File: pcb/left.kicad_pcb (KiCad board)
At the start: 2 copper layers, 1 part

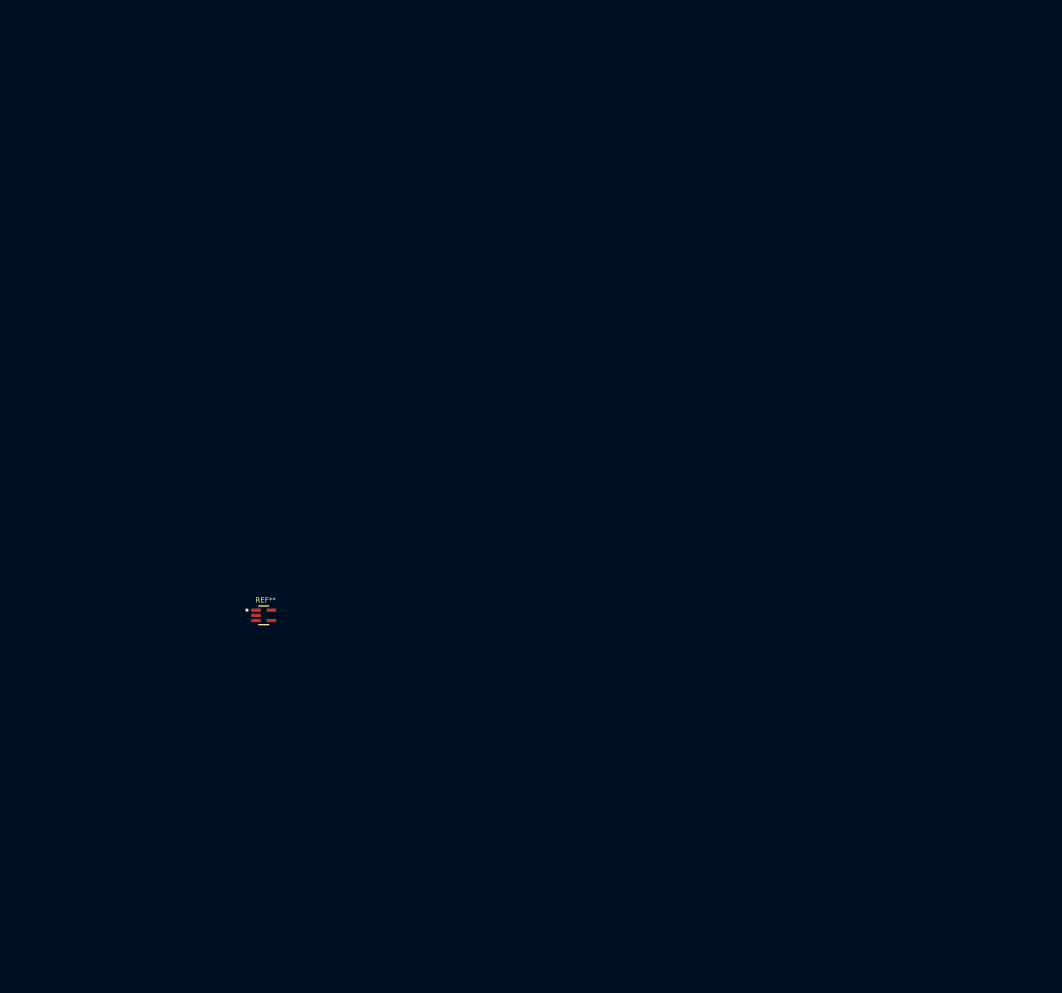
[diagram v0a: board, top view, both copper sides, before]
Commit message: close to finishing layout/placement
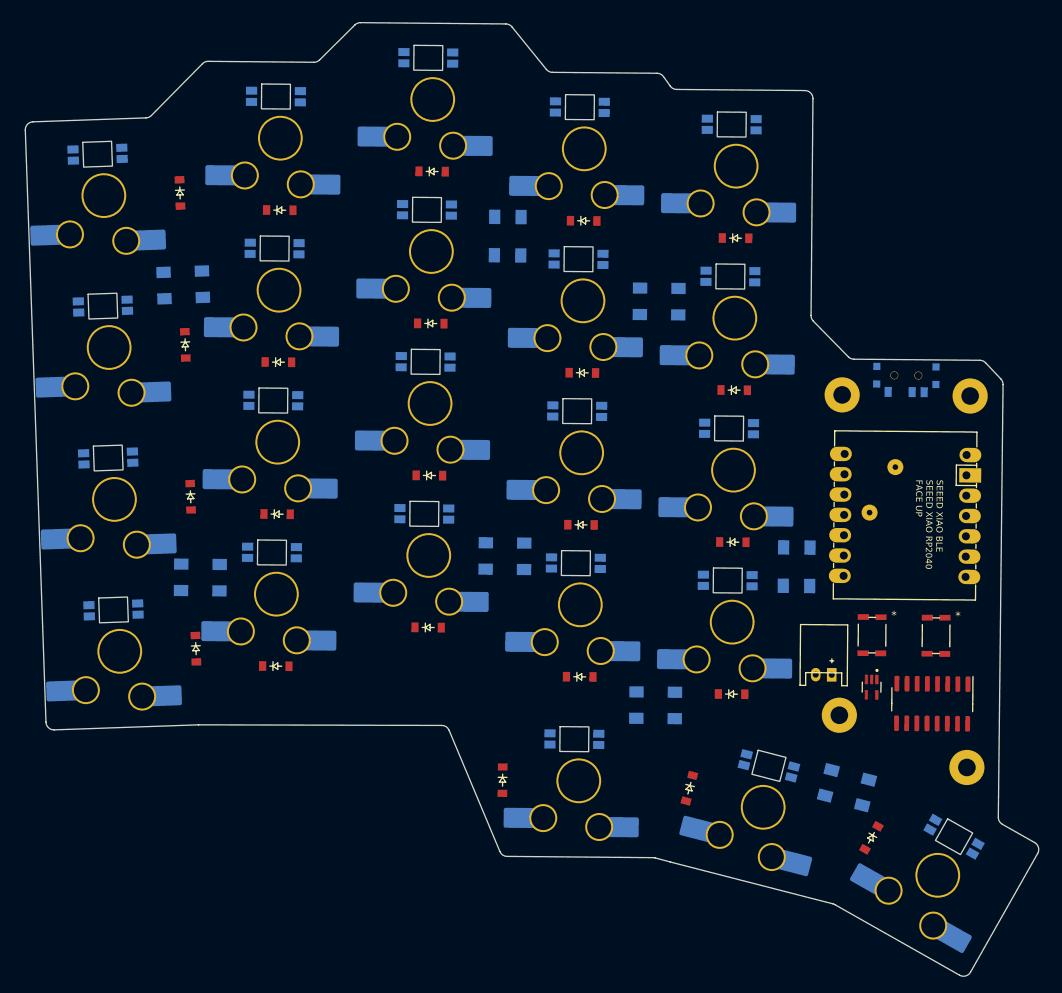
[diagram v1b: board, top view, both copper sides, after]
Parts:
- removed REF**: SOT65P210X110-5N, SN74LV1T34:SOT65P210X110-5N
- added 19.051: 74HC595, SOIC-16_3.9x9.9mm_P1.27mm, F.Cu at (201.6, 106.5)
- added D1: , ComboDiode, F.Cu at (119.5, 101.9)
- added D10: , ComboDiode, F.Cu at (157.7, 84.2)
- added D11: , ComboDiode, F.Cu at (157.8, 65.2)
- added D12: , ComboDiode, F.Cu at (158.0, 46.2)
- added D13: , ComboDiode, F.Cu at (176.5, 105.4)
- added D14: , ComboDiode, F.Cu at (176.6, 86.4)
- added D15: , ComboDiode, F.Cu at (176.8, 67.4)
- added D16: , ComboDiode, F.Cu at (177.0, 48.4)
- added D17: , ComboDiode, F.Cu at (147.9, 116.1)
- added D18: , ComboDiode, F.Cu at (171.2, 117.1)
- added D19: , ComboDiode, F.Cu at (194.0, 123.3)
- added D2: , ComboDiode, F.Cu at (119.7, 82.9)
- added D20: , ComboDiode, F.Cu at (109.5, 99.7)
- added D21: , ComboDiode, F.Cu at (108.9, 80.7)
- added D22: , ComboDiode, F.Cu at (108.2, 61.7)
- added D23: , ComboDiode, F.Cu at (107.5, 42.7)
- added D3: , ComboDiode, F.Cu at (119.8, 63.9)
- added D4: , ComboDiode, F.Cu at (120.0, 44.9)
- added D5: , ComboDiode, F.Cu at (138.5, 97.0)
- added D6: , ComboDiode, F.Cu at (138.7, 78.0)
- added D7: , ComboDiode, F.Cu at (138.9, 59.0)
- added D8: , ComboDiode, F.Cu at (139.0, 40.0)
- added D9: , ComboDiode, F.Cu at (157.5, 103.2)
- added JST1: , JST_PH_S2B-PH-K_02x2.00mm_Angled, F.Cu at (188.0, 102.9)
- added LED1: , ceoloide:led_SK6812mini-e (per-keysingle-side), B.Cu at (99.2, 94.8)
- added LED10: , ceoloide:led_SK6812mini-e (per-keysingle-side), B.Cu at (138.2, 63.8)
- added LED11: , ceoloide:led_SK6812mini-e (per-keysingle-side), B.Cu at (138.4, 44.8)
- added LED12: , ceoloide:led_SK6812mini-e (per-keysingle-side), B.Cu at (138.6, 25.8)
- added LED13: , ceoloide:led_SK6812mini-e (per-keysingle-side), B.Cu at (157.0, 89.0)
- added LED14: , ceoloide:led_SK6812mini-e (per-keysingle-side), B.Cu at (157.2, 70.0)
- added LED15: , ceoloide:led_SK6812mini-e (per-keysingle-side), B.Cu at (157.3, 51.0)
- added LED16: , ceoloide:led_SK6812mini-e (per-keysingle-side), B.Cu at (157.5, 32.0)
- added LED17: , ceoloide:led_SK6812mini-e (per-keysingle-side), B.Cu at (176.0, 91.1)
- added LED18: , ceoloide:led_SK6812mini-e (per-keysingle-side), B.Cu at (176.2, 72.1)
- added LED19: , ceoloide:led_SK6812mini-e (per-keysingle-side), B.Cu at (176.3, 53.1)
- added LED2: , ceoloide:led_SK6812mini-e (per-keysingle-side), B.Cu at (98.6, 75.8)
- added LED20: , ceoloide:led_SK6812mini-e (per-keysingle-side), B.Cu at (176.5, 34.1)
- added LED21: , ceoloide:led_SK6812mini-e (per-keysingle-side), B.Cu at (156.8, 111.0)
- added LED22: , ceoloide:led_SK6812mini-e (per-keysingle-side), B.Cu at (181.1, 114.3)
- added LED23: , ceoloide:led_SK6812mini-e (per-keysingle-side), B.Cu at (204.3, 123.2)
- added LED24: VAL**, WS2812B, B.Cu at (107.9, 54.2)
- added LED25: VAL**, WS2812B, B.Cu at (110.1, 90.8)
- added LED26: VAL**, WS2812B, B.Cu at (148.1, 88.1)
- added LED27: VAL**, WS2812B, B.Cu at (167.0, 106.7)
- added LED28: VAL**, WS2812B, B.Cu at (190.9, 117.0)
- added LED29: VAL**, WS2812B, B.Cu at (167.4, 56.3)
- added LED3: , ceoloide:led_SK6812mini-e (per-keysingle-side), B.Cu at (97.9, 56.8)
- added LED30: VAL**, WS2812B, B.Cu at (184.6, 89.4)
- added LED31: VAL**, WS2812B, B.Cu at (148.5, 48.1)
- added LED4: , ceoloide:led_SK6812mini-e (per-keysingle-side), B.Cu at (97.2, 37.9)
- added LED5: , ceoloide:led_SK6812mini-e (per-keysingle-side), B.Cu at (119.0, 87.6)
- added LED6: , ceoloide:led_SK6812mini-e (per-keysingle-side), B.Cu at (119.2, 68.6)
- added LED7: , ceoloide:led_SK6812mini-e (per-keysingle-side), B.Cu at (119.4, 49.7)
- added LED8: , ceoloide:led_SK6812mini-e (per-keysingle-side), B.Cu at (119.5, 30.7)
- added LED9: , ceoloide:led_SK6812mini-e (per-keysingle-side), B.Cu at (138.1, 82.8)
- added MCU1: , xiao-ble, F.Cu at (198.2, 83.0)
- added PAD1: , MountingHole_2.2mm_M2_Pad, F.Cu at (206.3, 68.1)
- added PAD2: , MountingHole_2.2mm_M2_Pad, F.Cu at (190.3, 67.9)
- added PAD3: , MountingHole_2.2mm_M2_Pad, F.Cu at (205.9, 114.5)
- added PAD4: , MountingHole_2.2mm_M2_Pad, F.Cu at (190.0, 108.0)
- added S1: , ceoloide:switch_gateron_ks27_ks33, B.Cu at (100.0, 100.0)
- added S10: , ceoloide:switch_gateron_ks27_ks33, B.Cu at (138.8, 69.0)
- added S11: , ceoloide:switch_gateron_ks27_ks33, B.Cu at (139.0, 50.0)
- added S12: , ceoloide:switch_gateron_ks27_ks33, B.Cu at (139.1, 31.0)
- added S13: , ceoloide:switch_gateron_ks27_ks33, B.Cu at (157.6, 94.2)
- added S14: , ceoloide:switch_gateron_ks27_ks33, B.Cu at (157.7, 75.2)
- added S15: , ceoloide:switch_gateron_ks27_ks33, B.Cu at (157.9, 56.2)
- added S16: , ceoloide:switch_gateron_ks27_ks33, B.Cu at (158.1, 37.2)
- added S17: , ceoloide:switch_gateron_ks27_ks33, B.Cu at (176.6, 96.4)
- added S18: , ceoloide:switch_gateron_ks27_ks33, B.Cu at (176.7, 77.4)
- added S19: , ceoloide:switch_gateron_ks27_ks33, B.Cu at (176.9, 58.4)
- added S2: , ceoloide:switch_gateron_ks27_ks33, B.Cu at (99.3, 81.0)
- added S20: , ceoloide:switch_gateron_ks27_ks33, B.Cu at (177.0, 39.4)
- added S21: , ceoloide:switch_gateron_ks27_ks33, B.Cu at (157.4, 116.2)
- added S22: , ceoloide:switch_gateron_ks27_ks33, B.Cu at (180.4, 119.5)
- added S23: , ceoloide:switch_gateron_ks27_ks33, B.Cu at (202.3, 128.0)
- added S3: , ceoloide:switch_gateron_ks27_ks33, B.Cu at (98.7, 62.0)
- added S4: , ceoloide:switch_gateron_ks27_ks33, B.Cu at (98.0, 43.0)
- added S5: , ceoloide:switch_gateron_ks27_ks33, B.Cu at (119.6, 92.9)
- added S6: , ceoloide:switch_gateron_ks27_ks33, B.Cu at (119.7, 73.9)
- added S7: , ceoloide:switch_gateron_ks27_ks33, B.Cu at (119.9, 54.9)
- added S8: , ceoloide:switch_gateron_ks27_ks33, B.Cu at (120.1, 35.9)
- added S9: , ceoloide:switch_gateron_ks27_ks33, B.Cu at (138.6, 88.0)
- added T1: , E73:SPDT_C128955, F.Cu at (198.3, 65.5)
- added _1: SOT65P210X110-5N, SOT65P210X110-5N, F.Cu at (194.0, 104.5)
- added _2: SMD_025816_WRE, SMD_025816_WRE, F.Cu at (194.0, 98.0)
- added _3: SMD_025816_WRE, SMD_025816_WRE, F.Cu at (202.0, 98.0)
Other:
- board outline added: 126.7 x 119.2 mm
- rule pad_to_mask_clearance: 0 -> 0.05

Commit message: trying to make mcu_cover
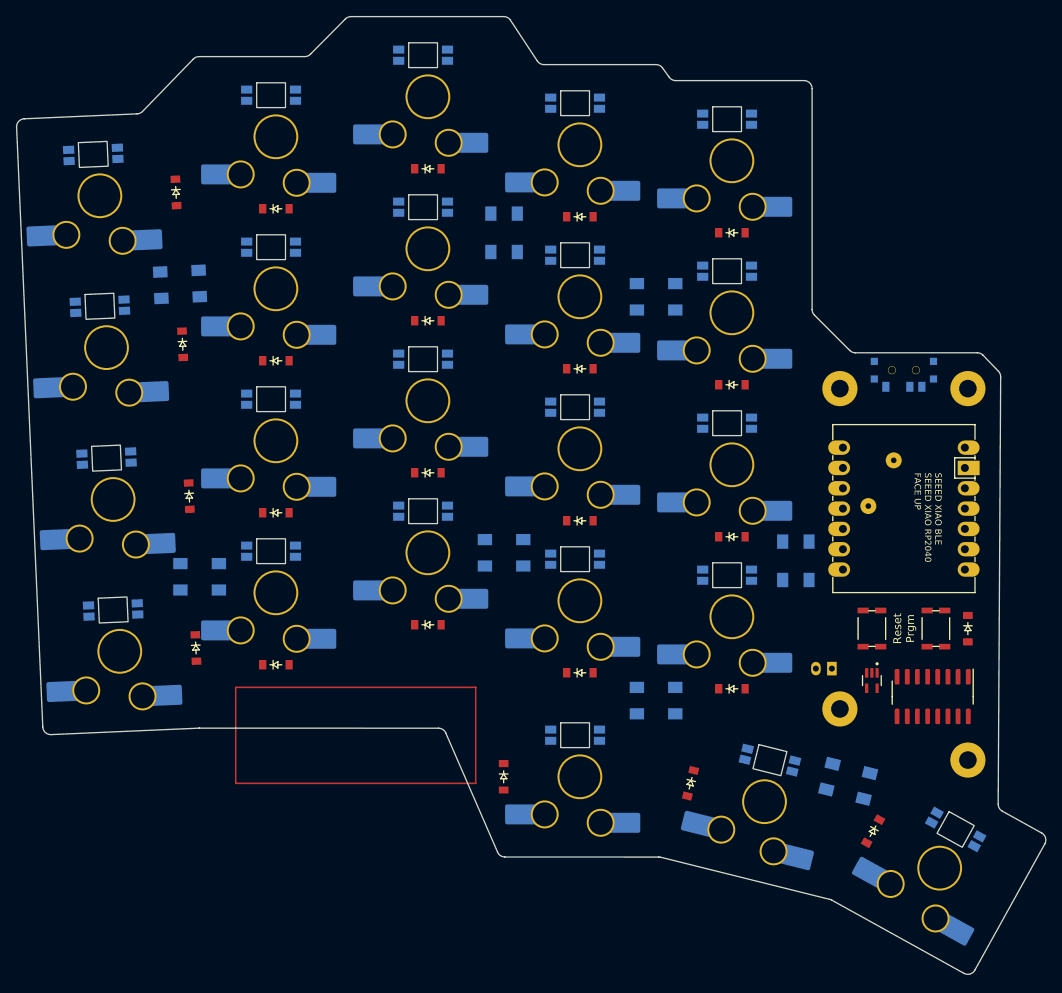
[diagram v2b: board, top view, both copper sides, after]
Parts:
- removed MCU1: , xiao-ble
- removed S1, S10, S11, S12, S13, S14, S15, S16, S17, S18, S19, S2, S20, S21, S22, S23, S3, S4, S5, S6, S7, S8, S9: , ceoloide:switch_gateron_ks27_ks33
- removed _1: SOT65P210X110-5N, SOT65P210X110-5N
- removed _2, _3: SMD_025816_WRE, SMD_025816_WRE
- added 19.052: 74HC595, SOIC-16_3.9x9.9mm_P1.27mm, F.Cu at (201.6, 105.7)
- added 19.053: SOT65P210X110-5N, SOT65P210X110-5N, F.Cu at (194.0, 103.7)
- added D24: , ComboDiode, F.Cu at (206.0, 97.2)
- added SW1: , ceoloide:switch_gateron_ks27_ks33, B.Cu at (100.0, 100.0)
- added SW10: , ceoloide:switch_gateron_ks27_ks33, B.Cu at (138.5, 68.7)
- added SW11: , ceoloide:switch_gateron_ks27_ks33, B.Cu at (138.5, 49.7)
- added SW12: , ceoloide:switch_gateron_ks27_ks33, B.Cu at (138.5, 30.7)
- added SW13: , ceoloide:switch_gateron_ks27_ks33, B.Cu at (157.5, 93.7)
- added SW14: , ceoloide:switch_gateron_ks27_ks33, B.Cu at (157.5, 74.7)
- added SW15: , ceoloide:switch_gateron_ks27_ks33, B.Cu at (157.5, 55.7)
- added SW16: , ceoloide:switch_gateron_ks27_ks33, B.Cu at (157.5, 36.7)
- added SW17: , ceoloide:switch_gateron_ks27_ks33, B.Cu at (176.5, 95.7)
- added SW18: , ceoloide:switch_gateron_ks27_ks33, B.Cu at (176.5, 76.7)
- added SW19: , ceoloide:switch_gateron_ks27_ks33, B.Cu at (176.5, 57.7)
- added SW2: , ceoloide:switch_gateron_ks27_ks33, B.Cu at (99.2, 81.0)
- added SW20: , ceoloide:switch_gateron_ks27_ks33, B.Cu at (176.5, 38.7)
- added SW21: , ceoloide:switch_gateron_ks27_ks33, B.Cu at (157.5, 115.7)
- added SW22: , ceoloide:switch_gateron_ks27_ks33, B.Cu at (180.6, 118.8)
- added SW23: , ceoloide:switch_gateron_ks27_ks33, B.Cu at (202.5, 127.1)
- added SW24: , SMD_025816_WRE, F.Cu at (202.0, 97.2)
- added SW25: , SMD_025816_WRE, F.Cu at (194.0, 97.2)
- added SW3: , ceoloide:switch_gateron_ks27_ks33, B.Cu at (98.3, 62.0)
- added SW4: , ceoloide:switch_gateron_ks27_ks33, B.Cu at (97.5, 43.1)
- added SW5: , ceoloide:switch_gateron_ks27_ks33, B.Cu at (119.5, 92.7)
- added SW6: , ceoloide:switch_gateron_ks27_ks33, B.Cu at (119.5, 73.7)
- added SW7: , ceoloide:switch_gateron_ks27_ks33, B.Cu at (119.5, 54.7)
- added SW8: , ceoloide:switch_gateron_ks27_ks33, B.Cu at (119.5, 35.7)
- added SW9: , ceoloide:switch_gateron_ks27_ks33, B.Cu at (138.5, 87.7)
- 19.051: value 74HC595 -> (none); footprint SOIC-16_3.9x9.9mm_P1.27mm -> xiao-ble
- moved 19.051 24.6 mm to (198.0, 82.2), turned to 0 degrees
- moved PAD1 0.97 mm to (206.0, 67.2), turned to 0 degrees
- moved PAD3 0.93 mm to (206.0, 113.6), turned to -29 degrees
- moved LED23 0.93 mm to (204.5, 122.3), turned to -29 degrees
- moved LED20 0.88 mm to (175.9, 33.5), turned to 0 degrees
- moved D19 0.84 mm to (194.2, 122.5), turned to -119 degrees
- moved PAD2 0.84 mm to (190.0, 67.2), turned to 0 degrees
- moved D16 0.81 mm to (176.5, 47.7), turned to 0 degrees
- moved LED28 0.81 mm to (191.0, 116.2), turned to -14 degrees
- moved PAD4 0.79 mm to (190.0, 107.2), turned to -14 degrees
- moved LED19 0.78 mm to (175.9, 52.5), turned to 0 degrees
- moved LED16 0.78 mm to (156.9, 31.5), turned to 0 degrees
- moved JST1 0.77 mm to (188.0, 102.2), turned to 180 degrees
- moved LED30 0.74 mm to (184.5, 88.7), turned to 90 degrees
- moved LED12 0.73 mm to (137.9, 25.5), turned to 0 degrees
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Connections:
- 19.051 pad 1: Col1 -> Row0
- 19.051 pad 10: VCC -> MISO
- 19.051 pad 11: SRCLK -> MOSI
- 19.051 pad 12: RCLK -> VCC
- 19.051 pad 14: SER -> 5v
- 19.051 pad 2: Col2 -> Row1
- 19.051 pad 3: Col3 -> Row2
- 19.051 pad 4: Col4 -> Row3
- 19.051 pad 5: QF -> Row4
- 19.051 pad 6: QG -> LED_3v3
- 19.051 pad 7: QH -> P6
- 19.051 pad 8: GND -> P7
- 19.051 pad 9: QH' -> SRCLK
- D1 pad 1: Row0 -> Row3
- D10 pad 1: Row1 -> Row2
- D11 pad 1: Row2 -> Row1
- D12 pad 1: Row3 -> Row0
- D13 pad 1: Row0 -> Row3
- D14 pad 1: Row1 -> Row2
- D15 pad 1: Row2 -> Row1
- D16 pad 1: Row3 -> Row0
- D2 pad 1: Row1 -> Row2
- D20 pad 1: Row0 -> Row3
- D21 pad 1: Row1 -> Row2
- D22 pad 1: Row2 -> Row1
- D23 pad 1: Row3 -> Row0
- D3 pad 1: Row2 -> Row1
- D4 pad 1: Row3 -> Row0
- D5 pad 1: Row0 -> Row3
- D6 pad 1: Row1 -> Row2
- D7 pad 1: Row2 -> Row1
- D8 pad 1: Row3 -> Row0
- D9 pad 1: Row0 -> Row3
- LED24 pad 1: (no net) -> 5v
- LED25 pad 1: (no net) -> 5v
- LED26 pad 1: (no net) -> 5v
- LED27 pad 1: (no net) -> 5v
- LED28 pad 1: (no net) -> 5v
- LED29 pad 1: (no net) -> 5v
- LED30 pad 1: (no net) -> 5v
- LED31 pad 1: (no net) -> 5v
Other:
- board size 126.7 x 119.2 mm -> 128.7 x 119.7 mm
